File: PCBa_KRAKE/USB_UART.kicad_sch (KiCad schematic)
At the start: 23 parts, among them J501 USB_C_Receptacle_USB2.0, Q205 MMBT2222A-7-F, U501 CH340B

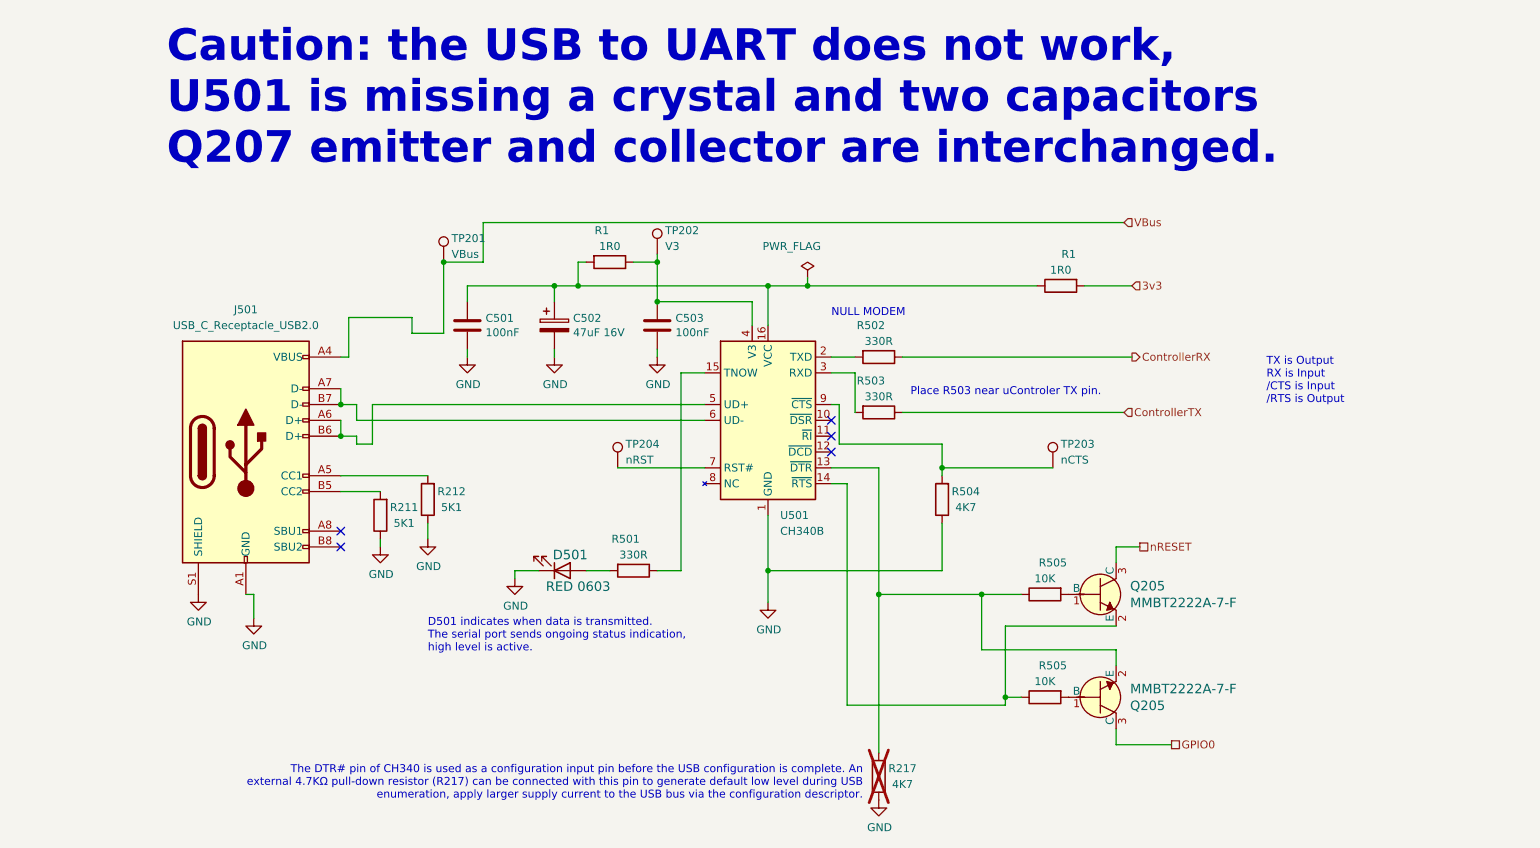
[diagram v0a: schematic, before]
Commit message: Fixed the previous PWA_REV_2 file by added the changes of the USB UART. PCBa_krake is reverted to when no changes done to the schem.
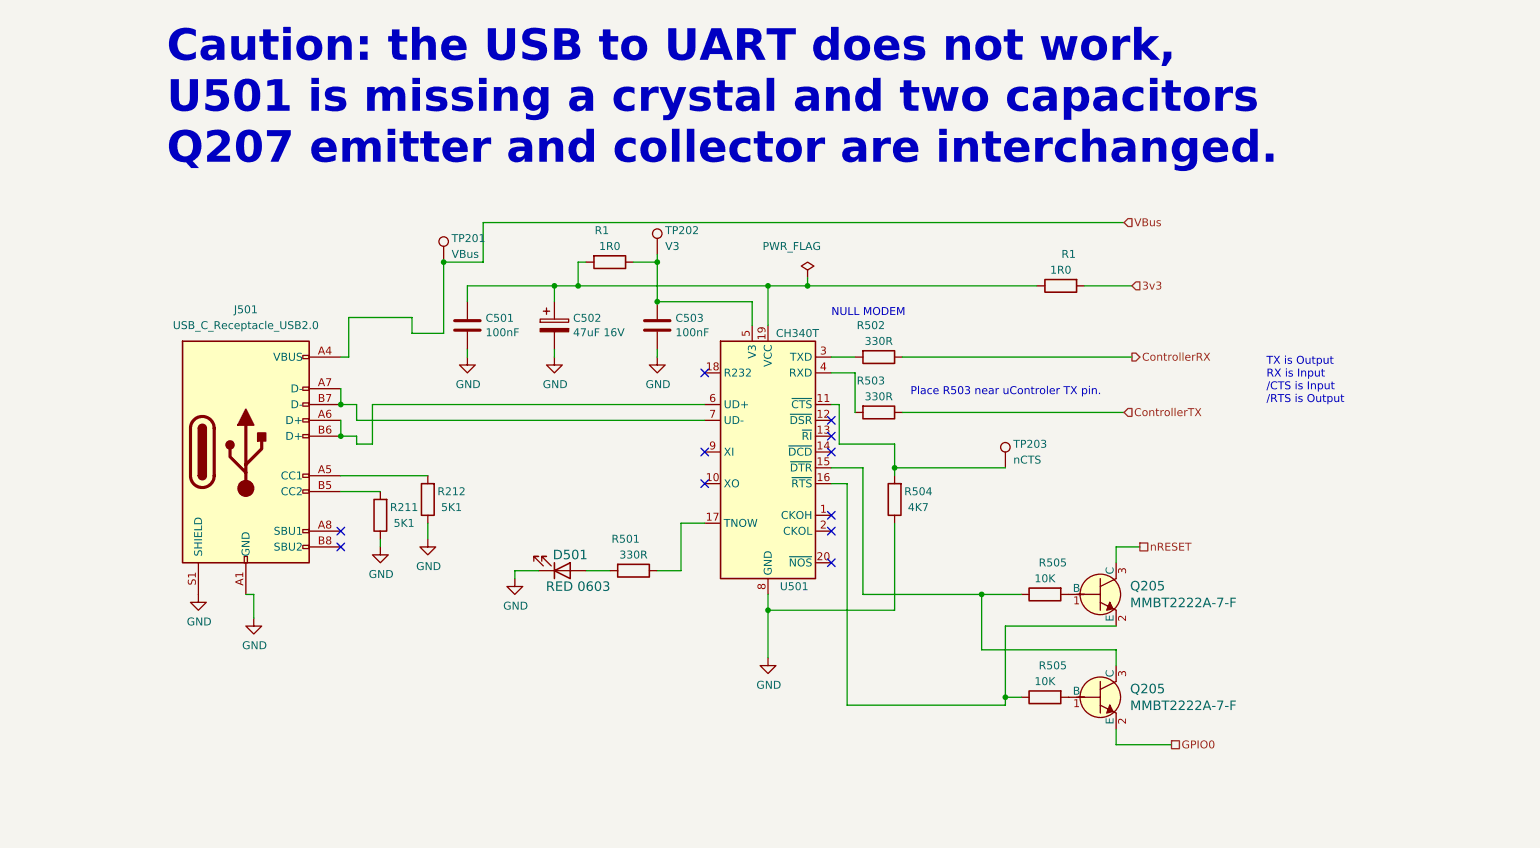
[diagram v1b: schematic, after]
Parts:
- removed R217: 4K7, Resistor_SMD:R_0603_1608Metric_Pad0.98x0.95mm_HandSolder, symbol Device:R
- removed TP204: nRST, TestPoint:TestPoint_Loop_D2.54mm_Drill1.5mm_Beaded, symbol Connector:TestPoint
- removed U501: CH340B, Package_SO:SOIC-16_3.9x9.9mm_P1.27mm, symbol GPAD_SCH_LIB:CH340B
- added U501: CH340T, GeneralPurposeAlarmDevicePCB:SSOP-20_5.3x7.2mm_P0.65mm_CH340T, symbol GPAD_SCH_LIB:CH340T
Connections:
- net GND: now also U501.8 (GND)
- net GPIO0: now also Q205.2 (E); no longer Q205.3 (C)
- net at R502.2: now also U501.3 (TXD)
- net at R503.2: now also U501.4 (RXD)
- net at C503.1, R1.1, TP202.1: now also U501.5 (V3)
- net at C501.1, C502.1, R1.1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: now also U501.19 (VCC)
- net at R501.1: now also U501.17 (TNOW)
- net at R504.2, TP203.1: now also U501.11 (~{CTS})
- net at R505.1: now also Q205.3 (C), U501.15 (~{DTR}); no longer Q205.2 (E)
- net at Q205.2 (E), R505.1: now also U501.16 (~{RTS})
- net at J501.A6 (D+), J501.B6 (D+): now also U501.6 (UD+)
- net at J501.A7 (D-), J501.B7 (D-): now also U501.7 (UD-)
- no-connect marks 5 -> 11
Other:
- note removed: "D501 indicates when data is transmitted. The serial port sends ongoing status indication, high level is active."
- note removed: "The DTR# pin of CH340 is used as a configuration input pin before the USB configuration is complete. An external 4.7KΩ pull-down resistor (R217) can be connected with this pin to generate default low level during USB enumeration, apply larger supply current to the USB bus via the configuration descriptor."
- moved on the sheet: R504, TP203
